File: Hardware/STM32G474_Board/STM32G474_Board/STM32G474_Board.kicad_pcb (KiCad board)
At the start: 2 copper layers, 1 part, among them CN1 NUCLEO (STM32G474RET6)

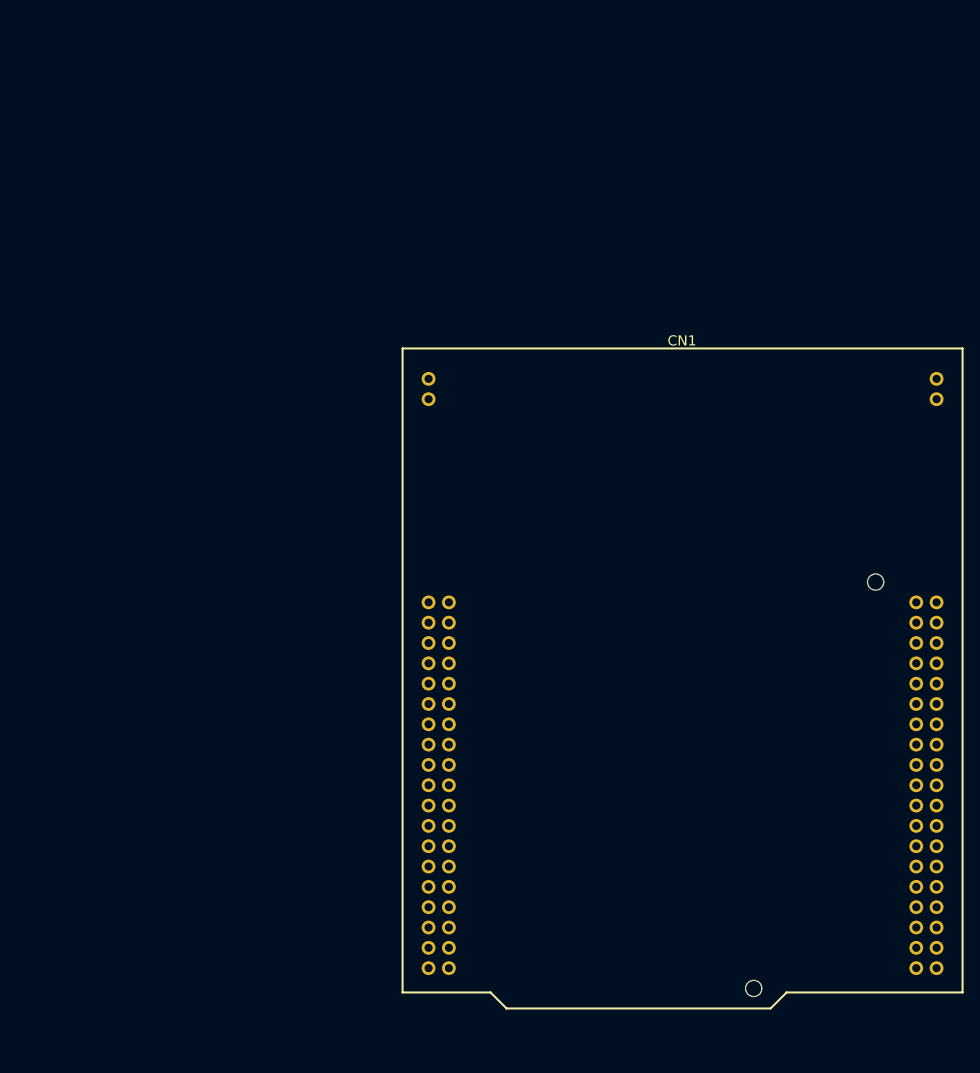
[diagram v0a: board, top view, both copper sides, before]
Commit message: Firmware
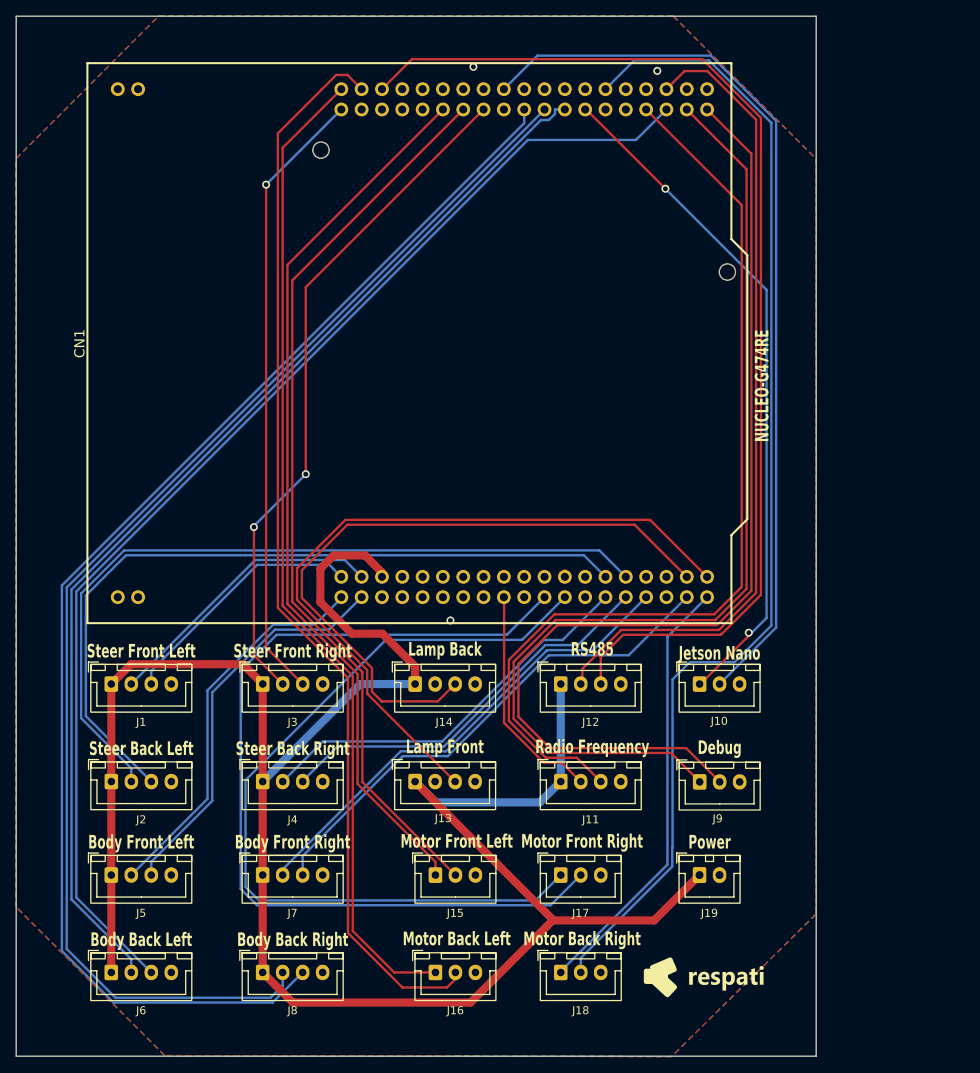
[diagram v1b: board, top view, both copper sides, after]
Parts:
- added G***: LOGO, LOGO, F.Cu at (100.4, 134.0)
- added J1: Steer_FL, Connector_JST:JST_XH_B4B-XH-A_1x04_P2.50mm_Vertical, F.Cu at (26.3, 97.4)
- added J10: Jetson, Connector_JST:JST_XH_B3B-XH-A_1x03_P2.50mm_Vertical, F.Cu at (99.9, 97.4)
- added J11: RF, Connector_JST:JST_XH_B4B-XH-A_1x04_P2.50mm_Vertical, F.Cu at (82.5, 109.5)
- added J12: RS485, Connector_JST:JST_XH_B4B-XH-A_1x04_P2.50mm_Vertical, F.Cu at (82.5, 97.4)
- added J13: Lamp_F, Connector_JST:JST_XH_B4B-XH-A_1x04_P2.50mm_Vertical, F.Cu at (64.3, 109.5)
- added J14: Lamp_B, Connector_JST:JST_XH_B4B-XH-A_1x04_P2.50mm_Vertical, F.Cu at (64.3, 97.4)
- added J15: Motor_FL, Connector_JST:JST_XH_B3B-XH-A_1x03_P2.50mm_Vertical, F.Cu at (66.8, 121.2)
- added J16: Motor_BL, Connector_JST:JST_XH_B3B-XH-A_1x03_P2.50mm_Vertical, F.Cu at (66.8, 133.4)
- added J17: Motor_FR, Connector_JST:JST_XH_B3B-XH-A_1x03_P2.50mm_Vertical, F.Cu at (82.5, 121.2)
- added J18: Motor_BR, Connector_JST:JST_XH_B3B-XH-A_1x03_P2.50mm_Vertical, F.Cu at (82.5, 133.4)
- added J19: Power, Connector_JST:JST_XH_B2B-XH-A_1x02_P2.50mm_Vertical, F.Cu at (99.8, 121.2)
- added J2: Steer_BL, Connector_JST:JST_XH_B4B-XH-A_1x04_P2.50mm_Vertical, F.Cu at (26.3, 109.5)
- added J3: Steer_FR, Connector_JST:JST_XH_B4B-XH-A_1x04_P2.50mm_Vertical, F.Cu at (45.2, 97.4)
- added J4: Steer_BR, Connector_JST:JST_XH_B4B-XH-A_1x04_P2.50mm_Vertical, F.Cu at (45.2, 109.5)
- added J5: Body_FL, Connector_JST:JST_XH_B4B-XH-A_1x04_P2.50mm_Vertical, F.Cu at (26.3, 121.2)
- added J6: Body_BL, Connector_JST:JST_XH_B4B-XH-A_1x04_P2.50mm_Vertical, F.Cu at (26.3, 133.4)
- added J7: Body_FR, Connector_JST:JST_XH_B4B-XH-A_1x04_P2.50mm_Vertical, F.Cu at (45.2, 121.2)
- added J8: Body_BR, Connector_JST:JST_XH_B4B-XH-A_1x04_P2.50mm_Vertical, F.Cu at (45.2, 133.4)
- added J9: Debug, Connector_JST:JST_XH_B3B-XH-A_1x03_P2.50mm_Vertical, F.Cu at (99.9, 109.6)
- moved CN1 64.6 mm to (105.8, 89.7), turned to 90 degrees
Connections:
- CN1 pad 1: unconnected-(CN1-PC10-Pad1) -> LinearL_4
- CN1 pad 13: T_SWDIO -> unconnected-(CN1-PA13-Pad13)
- CN1 pad 15: T_SWCLK -> unconnected-(CN1-PA14-Pad15)
- CN1 pad 19: unconnected-(CN1-GND-Pad19) -> GND
- CN1 pad 2: unconnected-(CN1-PC11-Pad2) -> LinearR_0
- CN1 pad 20: unconnected-(CN1-GND-Pad20) -> GND
- CN1 pad 22: unconnected-(CN1-GND-Pad22) -> GND
- CN1 pad 23: unconnected-(CN1-PC13-Pad23) -> MotorS_1
- CN1 pad 27: unconnected-(CN1-PC15-Pad27) -> LinearL_3
- CN1 pad 28: MotorS_0 -> LinearR_2
- CN1 pad 29: unconnected-(CN1-PF0-Pad29) -> LinearR_3
- CN1 pad 3: unconnected-(CN1-PC12-Pad3) -> LinearR_4
- CN1 pad 30: MotorS_1 -> LinearL_2
- CN1 pad 31: unconnected-(CN1-PF1-Pad31) -> LinearL_5
- CN1 pad 32: LinearR_11 -> unconnected-(CN1-PA4-Pad32)
- CN1 pad 34: LED_Jetson -> unconnected-(CN1-PB0-Pad34)
- CN1 pad 35: unconnected-(CN1-PC2-Pad35) -> LinearR_5
- CN1 pad 36: unconnected-(CN1-PB9/PC1_(PC1)-Pad36) -> Lamp_B
- CN1 pad 37: unconnected-(CN1-PC3-Pad37) -> MotorS_3
- CN1 pad 38: unconnected-(CN1-PA15/PC0_(PC0)-Pad38) -> Lamp_F
- CN1 pad 39: unconnected-(CN1-PC9-Pad39) -> LinearR_1
- CN1 pad 4: unconnected-(CN1-PD2-Pad4) -> LinearL_0
- CN1 pad 40: unconnected-(CN1-PC8-Pad40) -> MotorS_2
- CN1 pad 42: unconnected-(CN1-PC6-Pad42) -> MotorP_2
- CN1 pad 43: LinearL_11 -> unconnected-(CN1-PB9-Pad43)
- CN1 pad 44: unconnected-(CN1-PC5-Pad44) -> RS485_RX
- CN1 pad 47: unconnected-(CN1-GND-Pad47) -> GND
- CN1 pad 49: LinearL_5 -> MotorS_0
- CN1 pad 53: LinearR_6 -> LinearL_1
- CN1 pad 54: LinearR_8 -> unconnected-(CN1-PB12-Pad54)
- CN1 pad 55: LinearL_10 -> unconnected-(CN1-PB6-Pad55)
- CN1 pad 57: unconnected-(CN1-PC7-Pad57) -> LinearR_7
- CN1 pad 58: unconnected-(CN1-GND-Pad58) -> GND
- CN1 pad 59: LinearR_7 -> LinearL_7
- CN1 pad 6: unconnected-(CN1-E5V-Pad6) -> +5V
- CN1 pad 60: LED_Heartbeat -> unconnected-(CN1-PB2-Pad60)
- CN1 pad 62: LED_RF -> unconnected-(CN1-PB1-Pad62)
- CN1 pad 64: LinearR_9 -> unconnected-(CN1-PB15-Pad64)
- CN1 pad 65: LinearL_9 -> unconnected-(CN1-PB4-Pad65)
- CN1 pad 67: LinearR_10 -> unconnected-(CN1-PB5-Pad67)
- CN1 pad 68: LinearL_8 -> unconnected-(CN1-PB13-Pad68)
- CN1 pad 7: (BOOT0) -> unconnected-(CN1-PB8-BOOT0-Pad7)
- CN1 pad 70: unconnected-(CN1-AGND-Pad70) -> GND
- CN1 pad 71: LinearL_7 -> LinearR_6
- CN1 pad 72: unconnected-(CN1-PC4-Pad72) -> RS485_TX
- CN1 pad 8: unconnected-(CN1-GND-Pad8) -> GND
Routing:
- net +5V: track 0.00 -> 269.5 mm
- net LinearR_7: track 0.00 -> 163.4 mm
- net LinearL_7: track 0.00 -> 161.5 mm
- net LinearR_6: track 0.00 -> 150.2 mm
- net MotorP_3: track 0.00 -> 145.0 mm
- net RS485_RX: track 0.00 -> 138.2 mm
- net LinearL_6: track 0.00 -> 137.8 mm
- net MotorP_2: track 0.00 -> 135.3 mm
- net Debug_RX: track 0.00 -> 130.5 mm
- net Debug_TX: track 0.00 -> 129.5 mm
- net MotorS_2: track 0.00 -> 124.7 mm
- net RF_TX: track 0.00 -> 119.8 mm
- net MotorP_1: track 0.00 -> 114.0 mm
- net MotorP_0: track 0.00 -> 113.0 mm
- net Jetson_RX: track 0.00 -> 112.5 mm
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- added copper zone on B.Cu, net GND
- added copper zone on F.Cu, net GND
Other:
- board outline added: 100 x 130 mm
- board text added: "Body Back Left"
- board text added: "Body Back Right"
- board text added: "Body Front Left"
- board text added: "Body Front Right"
- board text added: "Debug"
- board text added: "Jetson Nano"
- board text added: "Lamp Back"
- board text added: "Lamp Front"
- board text added: "Motor Back Left"
- board text added: "Motor Back Right"
- board text added: "Motor Front Left"
- board text added: "Motor Front Right"
- board text added: "NUCLEO-G474RE"
- board text added: "Power"
- board text added: "RS485"
- board text added: "Radio Frequency"
- board text added: "Steer Back Left"
- board text added: "Steer Back Right"
- board text added: "Steer Front Left"
- board text added: "Steer Front Right"
